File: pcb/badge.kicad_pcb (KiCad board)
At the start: 2 copper layers, 35 x 22 mm, 26 parts, among them IC102 AAT3681A, P1 CONN_01X04, P102 CONN_01X02, P103 USB_OTG, P2 CONNECTOR, P3 CONNECTOR, Q1 NPN, Q101 FT230XS-R, Q102 NPN

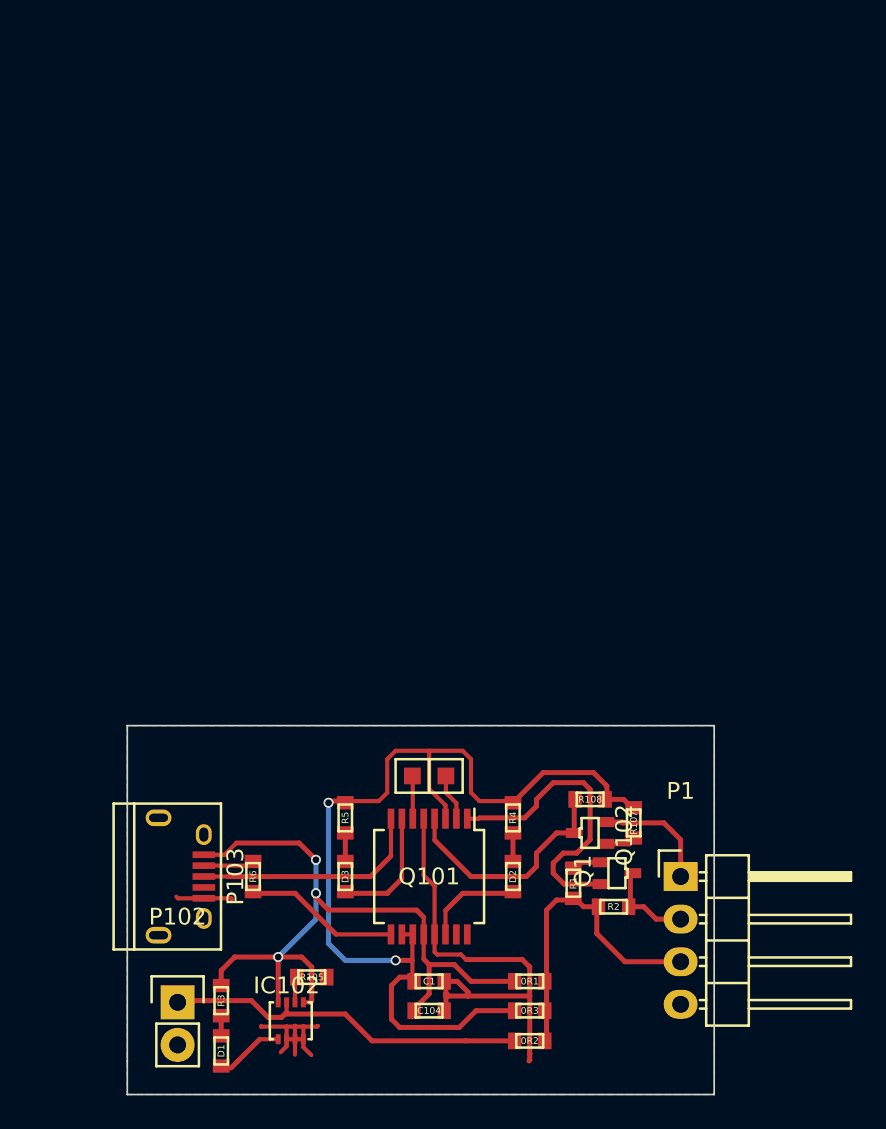
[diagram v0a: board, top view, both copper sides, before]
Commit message: first complete version
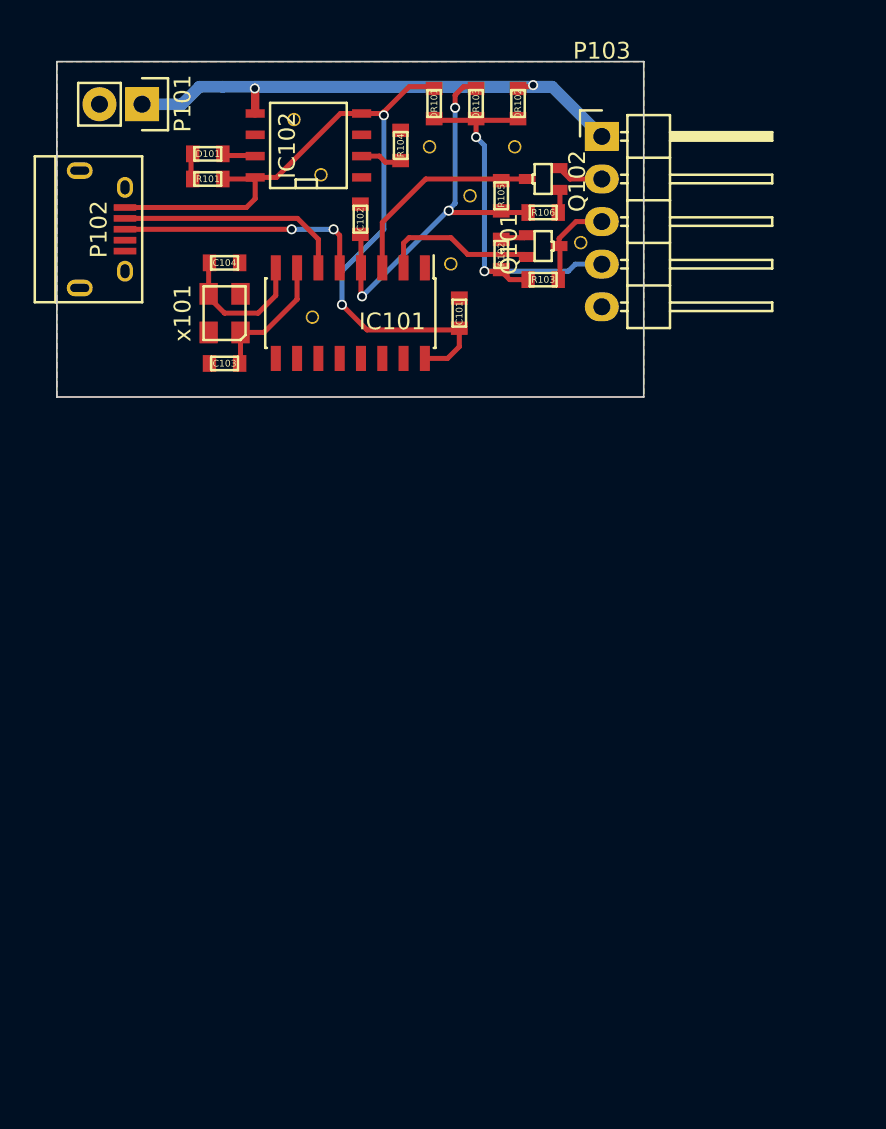
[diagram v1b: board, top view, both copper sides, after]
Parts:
- removed 0R1, 0R2, 0R3, R1, R107, R108, R2, R3, R4, R5: R, netl:SMD_0603
- removed C1: 10u, netl:SMD_0603
- removed D1, D2, D3: LED, netl:SMD_0603
- removed P1: CONN_01X04, Pin_Headers:Pin_Header_Angled_1x04
- removed P2, P3: CONNECTOR, netl:1Pin_small
- removed Q1: NPN, TO_SOT_Packages_SMD:SOT-323
- removed R6: 0R, netl:SMD_0603
- added 0R101: R, netl:SMD_0603, F.Cu at (137.5, 72.5)
- added 0R102: R, netl:SMD_0603, F.Cu at (142.5, 72.5)
- added 0R103: R, netl:SMD_0603, F.Cu at (140.0, 72.5)
- added C101: 10u, netl:SMD_0603, F.Cu at (139.0, 85.0)
- added C102: 10u, netl:SMD_0603, F.Cu at (133.1, 79.4)
- added C103: C, netl:SMD_0603, F.Cu at (125.0, 88.0)
- added D101: LED, netl:SMD_0603, F.Cu at (124.0, 75.5)
- added G***: LOGO, netl:LOGO_127mm_Bottom_SS, F.Cu at (132.5, 80.0)
- added IC101: CH340G, Housings_SOIC:SOIC-16_3.9x9.9mm_Pitch1.27mm, F.Cu at (132.5, 85.0)
- added P101: CONN_01X02, Pin_Headers:Pin_Header_Straight_1x02, F.Cu at (120.1, 72.5)
- added R101: R, netl:SMD_0603, F.Cu at (124.0, 77.0)
- added R102: R, netl:SMD_0603, F.Cu at (141.5, 81.5)
- added R103: R, netl:SMD_0603, F.Cu at (144.0, 83.0)
- added R104: R, netl:SMD_0603, F.Cu at (135.5, 75.0)
- added R106: R, netl:SMD_0603, F.Cu at (144.0, 79.0)
- added REF**: via, netl:via, F.Cu at (129.1, 73.5)
- added REF**: via, netl:via, F.Cu at (130.2, 85.2)
- added REF**: via, netl:via, F.Cu at (146.2, 80.8)
- added REF**: via, netl:via, F.Cu at (142.3, 75.1)
- added REF**: via, netl:via, F.Cu at (137.2, 75.1)
- added REF**: via, netl:via, F.Cu at (139.6, 78.0)
- added REF**: via, netl:via, F.Cu at (138.5, 82.1)
- added REF**: via, netl:via, F.Cu at (130.8, 76.8)
- added x101: xtal_osc, netl:SM_3225, F.Cu at (125.0, 85.0)
- C104: value 10u -> C
- IC102: value AAT3681A -> TP4056; footprint netl:SC70JW-8 -> SMD_Packages:SOIC-8-N
- P102: value CONN_01X02 -> USB_OTG; footprint Pin_Headers:Pin_Header_Straight_1x02 -> Connect:USB_Micro-B
- P103: value USB_OTG -> CONN_01X05; footprint Connect:USB_Micro-B -> Pin_Headers:Pin_Header_Angled_1x05
- Q101: value FT230XS-R -> NPN; footprint Housings_SSOP:SSOP-16_5.3x6.2mm_Pitch0.65mm -> TO_SOT_Packages_SMD:SOT-323
- moved IC102 51.1 mm to (130.0, 75.0), turned to 90 degrees
- moved P103 50.9 mm to (147.5, 74.5), turned to 0 degrees
- moved R105 48.0 mm to (141.5, 78.0), turned to 90 degrees
- moved P102 46.3 mm to (117.5, 80.0), turned to 270 degrees
- moved C104 46.2 mm to (125.0, 82.0)
- moved Q102 39.1 mm to (144.0, 77.0)
- moved Q101 38.2 mm to (144.0, 81.0), turned to 90 degrees
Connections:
- C104 pad 1: V_USB -> Net-(C104-Pad1)
- IC102 pad 1: V_USB -> (no net)
- IC102 pad 3: VBat -> GND
- IC102 pad 5: chrg -> VBat
- IC102 pad 6: GND -> (no net)
- IC102 pad 7: GND -> Net-(D101-Pad1)
- IC102 pad 8: GND -> V_USB
- P102 pad 1: VBat -> V_USB
- P102 pad 2: GND -> D-
- P103 pad 1: V_USB -> VBat
- P103 pad 2: Net-(P103-Pad2) -> AVR_TX
- P103 pad 3: D+ -> AVR_RX
- P103 pad 4: Net-(P103-Pad4) -> AVR_VCC
- Q101 pad 2: Net-(P2-Pad1) -> TX
- Q101 pad 3: 3V3 -> AVR_RX
- Q102 pad 3: Net-(Q101-Pad4) -> RX
- R105 pad 1: Net-(IC102-Pad2) -> 3V3
- R105 pad 2: GND -> RX
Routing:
- net GND: track 42.0 -> 0.16 mm
- net 3V3: track 57.9 -> 24.4 mm, vias 2 -> 3
- net VBat: track 21.9 -> 50.4 mm, vias 0 -> 2
- net Net-(Q101-Pad1): track 18.1 -> 1.61 mm
- net Net-(Q101-Pad4): track 14.1 -> 0.00 mm
- net RX: track 0.00 -> 12.4 mm
- net Net-(C104-Pad1): track 0.00 -> 9.55 mm
- net TX: track 0.00 -> 9.46 mm
- net Net-(C103-Pad1): track 0.00 -> 7.94 mm
- net Net-(D3-Pad1): track 7.31 -> 0.00 mm
- net Net-(D2-Pad1): track 5.87 -> 0.00 mm
- net AVR_VCC: track 18.5 -> 24.1 mm, vias 0 -> 2
- net D-: track 9.24 -> 13.8 mm
- net AVR_TX: track 7.09 -> 2.82 mm
- net chrg: track 4.10 -> 0.00 mm
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- added copper zone on B.Cu, net GND
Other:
- board size 35 x 22 mm -> 35 x 20 mm
